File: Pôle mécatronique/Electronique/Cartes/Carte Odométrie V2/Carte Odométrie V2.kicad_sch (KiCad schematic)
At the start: 32 parts, among them J1 Conn_01x03, J2 Conn_01x03, J3 Conn_01x03, U1 MCP2551-I-P

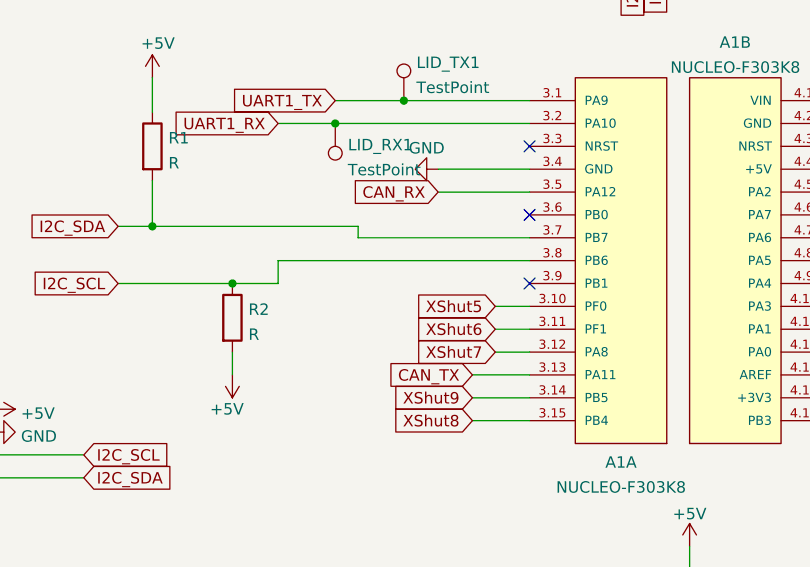
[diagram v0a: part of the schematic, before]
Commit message: Carte odo
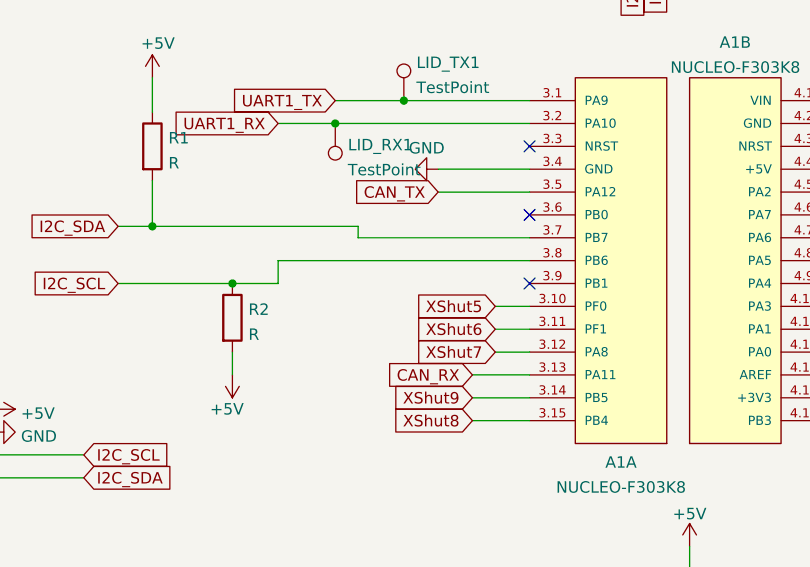
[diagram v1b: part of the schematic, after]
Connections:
- net CAN_RX: now also A1.3.13 (PA11); no longer A1.3.5 (PA12)
- net CAN_TX: now also A1.3.5 (PA12); no longer A1.3.13 (PA11)
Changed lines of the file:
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@@
+    (stroke (width 0) (type default) (color 0 0 0 0))
+  )
+  (wire (pts (xy 167.64 62.23) (xy 173.99 62.23))
+    (stroke (width 0) (type default) (color 0 0 0 0))
+  )
+  (wire (pts (xy 105.41 76.2) (xy 105.41 74.93))
+    (stroke (width 0) (type default) (color 0 0 0 0))
+  )
+  (wire (pts (xy 157.48 73.66) (xy 163.83 73.66))
+    (stroke (width 0) (type default) (color 0 0 0 0))
+  )
+  (wire (pts (xy 135.89 38.1) (xy 135.89 41.91))
+    (stroke (width 0) (type default) (color 0 0 0 0))
+  )
+  (wire (pts (xy 228.6 66.04) (xy 237.49 66.04))
+    (stroke (width 0) (type default) (color 0 0 0 0))
+  )
+  (wire (pts (xy 213.36 88.9) (xy 215.9 88.9))
+    (stroke (width 0) (type default) (color 0 0 0 0))
+  )
+  (wire (pts (xy 58.42 100.33) (xy 74.93 100.33))
     (stroke (width 0) (type default) (color 0 0 0 0))
   )
@@
     (stroke (width 0) (type default) (color 0 0 0 0))
   )
-  (wire (pts (xy 167.64 62.23) (xy 173.99 62.23))
-    (stroke (width 0) (type default) (color 0 0 0 0))
-  )
-  (wire (pts (xy 105.41 76.2) (xy 105.41 74.93))
-    (stroke (width 0) (type default) (color 0 0 0 0))
-  )
-  (wire (pts (xy 157.48 73.66) (xy 163.83 73.66))
-    (stroke (width 0) (type default) (color 0 0 0 0))
-  )
-  (wire (pts (xy 135.89 38.1) (xy 135.89 41.91))
-    (stroke (width 0) (type default) (color 0 0 0 0))
-  )
-  (wire (pts (xy 228.6 66.04) (xy 237.49 66.04))
-    (stroke (width 0) (type default) (color 0 0 0 0))
-  )
-  (wire (pts (xy 213.36 88.9) (xy 215.9 88.9))
-    (stroke (width 0) (type default) (color 0 0 0 0))
-  )
-  (wire (pts (xy 58.42 100.33) (xy 74.93 100.33))
-    (stroke (width 0) (type default) (color 0 0 0 0))
-  )
   (wire (pts (xy 125.73 144.78) (xy 129.54 144.78))
     (stroke (width 0) (type default) (color 0 0 0 0))
@@
     )
   )
-  (global_label "CAN_TX" (shape input) (at 118.11 91.44 180) (fields_autoplaced)
-    (effects (font (size 1.27 1.27)) (justify right))
-    (property "Intersheet References" "${INTERSHEET_REFS}" (id 0) (at 108.952 91.3606 0)
+  (global_label "CAN_TX" (shape input) (at 114.3 71.12 180) (fields_autoplaced)
+    (effects (font (size 1.27 1.27)) (justify right))
+    (property "Intersheet References" "${INTERSHEET_REFS}" (id 0) (at 105.142 71.0406 0)
       (effects (font (size 1.27 1.27)) (justify right) hide)
     )
@@
     )
   )
-  (global_label "CAN_RX" (shape input) (at 114.3 71.12 180) (fields_autoplaced)
-    (effects (font (size 1.27 1.27)) (justify right))
-    (property "Intersheet References" "${INTERSHEET_REFS}" (id 0) (at 104.8396 71.0406 0)
-      (effects (font (size 1.27 1.27)) (justify right) hide)
-    )
-  )
   (global_label "CAN_H" (shape input) (at 215.9 36.83 180) (fields_autoplaced)
     (effects (font (size 1.27 1.27)) (justify right))
@@
     )
   )
+  (global_label "CAN_RX" (shape input) (at 118.11 91.44 180) (fields_autoplaced)
+    (effects (font (size 1.27 1.27)) (justify right))
+    (property "Intersheet References" "${INTERSHEET_REFS}" (id 0) (at 108.6496 91.3606 0)
+      (effects (font (size 1.27 1.27)) (justify right) hide)
+    )
+  )

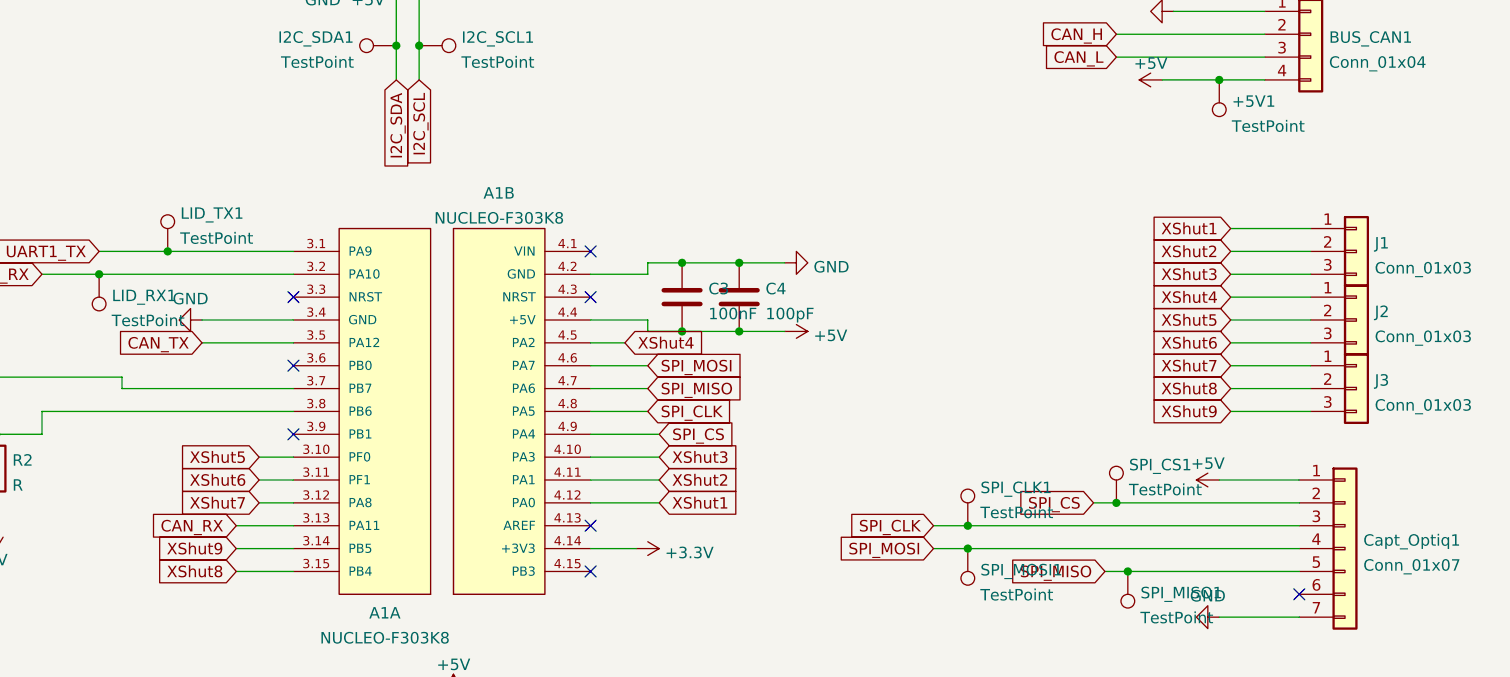
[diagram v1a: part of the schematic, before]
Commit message: Update Araignée & Odométrie
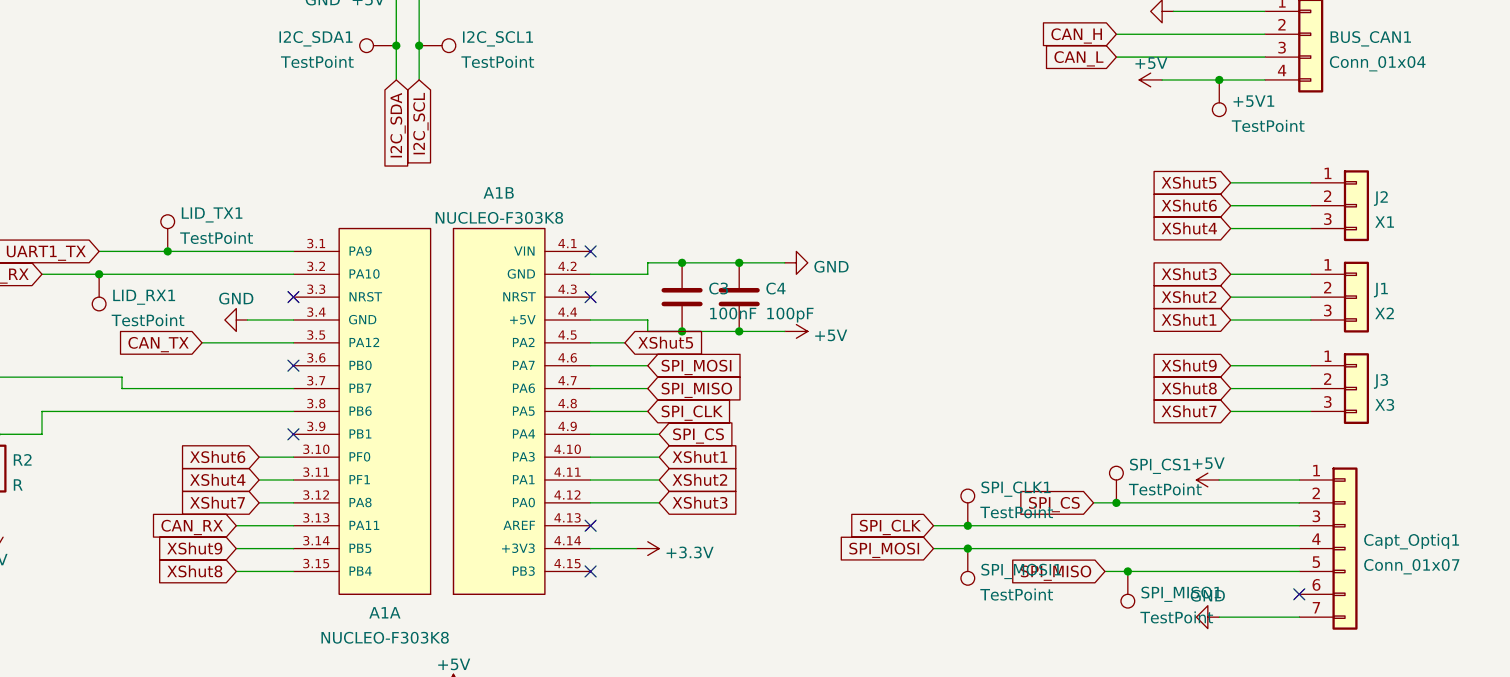
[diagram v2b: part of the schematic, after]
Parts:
- J1: value Conn_01x03 -> X2
- J2: value Conn_01x03 -> X1
- J3: value Conn_01x03 -> X3
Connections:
- net XShut1: now also A1.4.10 (PA3), J1.3 (Pin_3); no longer A1.4.12 (PA0), J1.1 (Pin_1)
- net XShut3: now also A1.4.12 (PA0), J1.1 (Pin_1); no longer A1.4.10 (PA3), J1.3 (Pin_3)
- net XShut4: now also A1.3.11 (PF1), J2.3 (Pin_3); no longer A1.4.5 (PA2), J2.1 (Pin_1)
- net XShut5: now also A1.4.5 (PA2), J2.1 (Pin_1); no longer A1.3.10 (PF0), J2.2 (Pin_2)
- net XShut6: now also A1.3.10 (PF0), J2.2 (Pin_2); no longer A1.3.11 (PF1), J2.3 (Pin_3)
- net XShut7: now also J3.3 (Pin_3); no longer J3.1 (Pin_1)
- net XShut9: now also J3.1 (Pin_1); no longer J3.3 (Pin_3)
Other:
- moved on the sheet: J1, J2

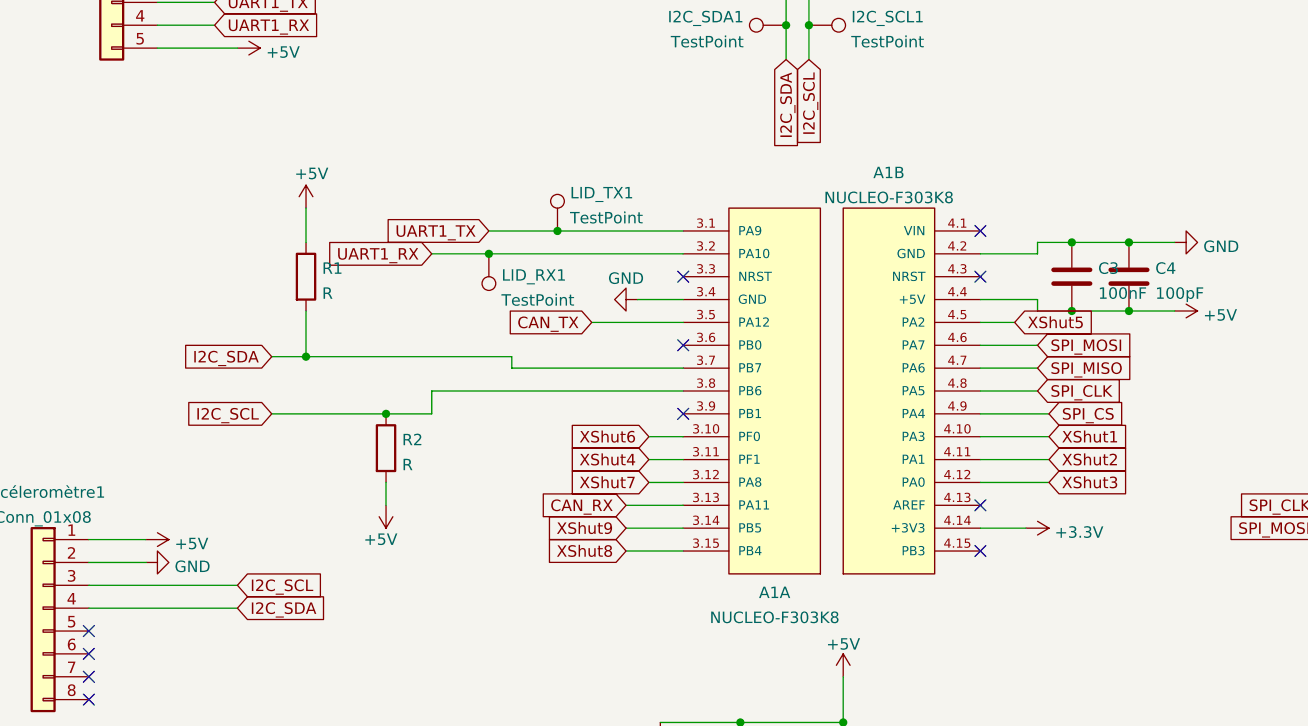
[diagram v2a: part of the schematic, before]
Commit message: Panique totale
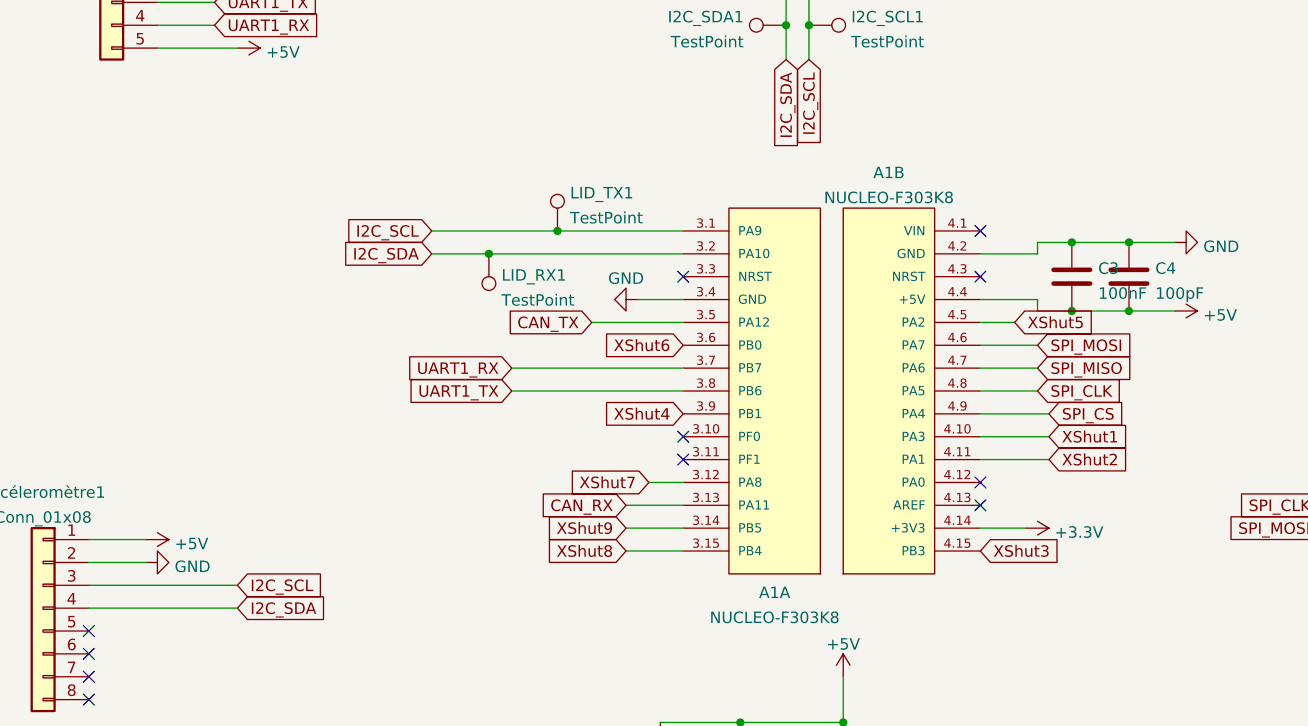
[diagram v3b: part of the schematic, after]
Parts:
- removed R1, R2: R, Resistor_THT:R_Axial_DIN0207_L6.3mm_D2.5mm_P10.16mm_Horizontal, symbol Device:R
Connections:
- net I2C_SCL: now also A1.3.1 (PA9), LID_TX1.1; no longer A1.3.8 (PB6)
- net I2C_SDA: now also A1.3.2 (PA10), LID_RX1.1; no longer A1.3.7 (PB7)
- net UART1_RX: now also A1.3.7 (PB7); no longer A1.3.2 (PA10), LID_RX1.1
- net UART1_TX: now also A1.3.8 (PB6); no longer A1.3.1 (PA9), LID_TX1.1
- net XShut3: now also A1.4.15 (PB3); no longer A1.4.12 (PA0)
- net XShut4: now also A1.3.9 (PB1); no longer A1.3.11 (PF1)
- net XShut6: now also A1.3.6 (PB0); no longer A1.3.10 (PF0)
